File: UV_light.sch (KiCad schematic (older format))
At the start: 89 parts, among them P1 SMD_CONN, P10 SMD_CONN, P2 SMD_CONN, P3 SMD_CONN, P4 SMD_CONN, P5 CONN_01X01, P6 CONN_01X01, P7 SMD_CONN, P8 SMD_CONN, P9 SMD_CONN

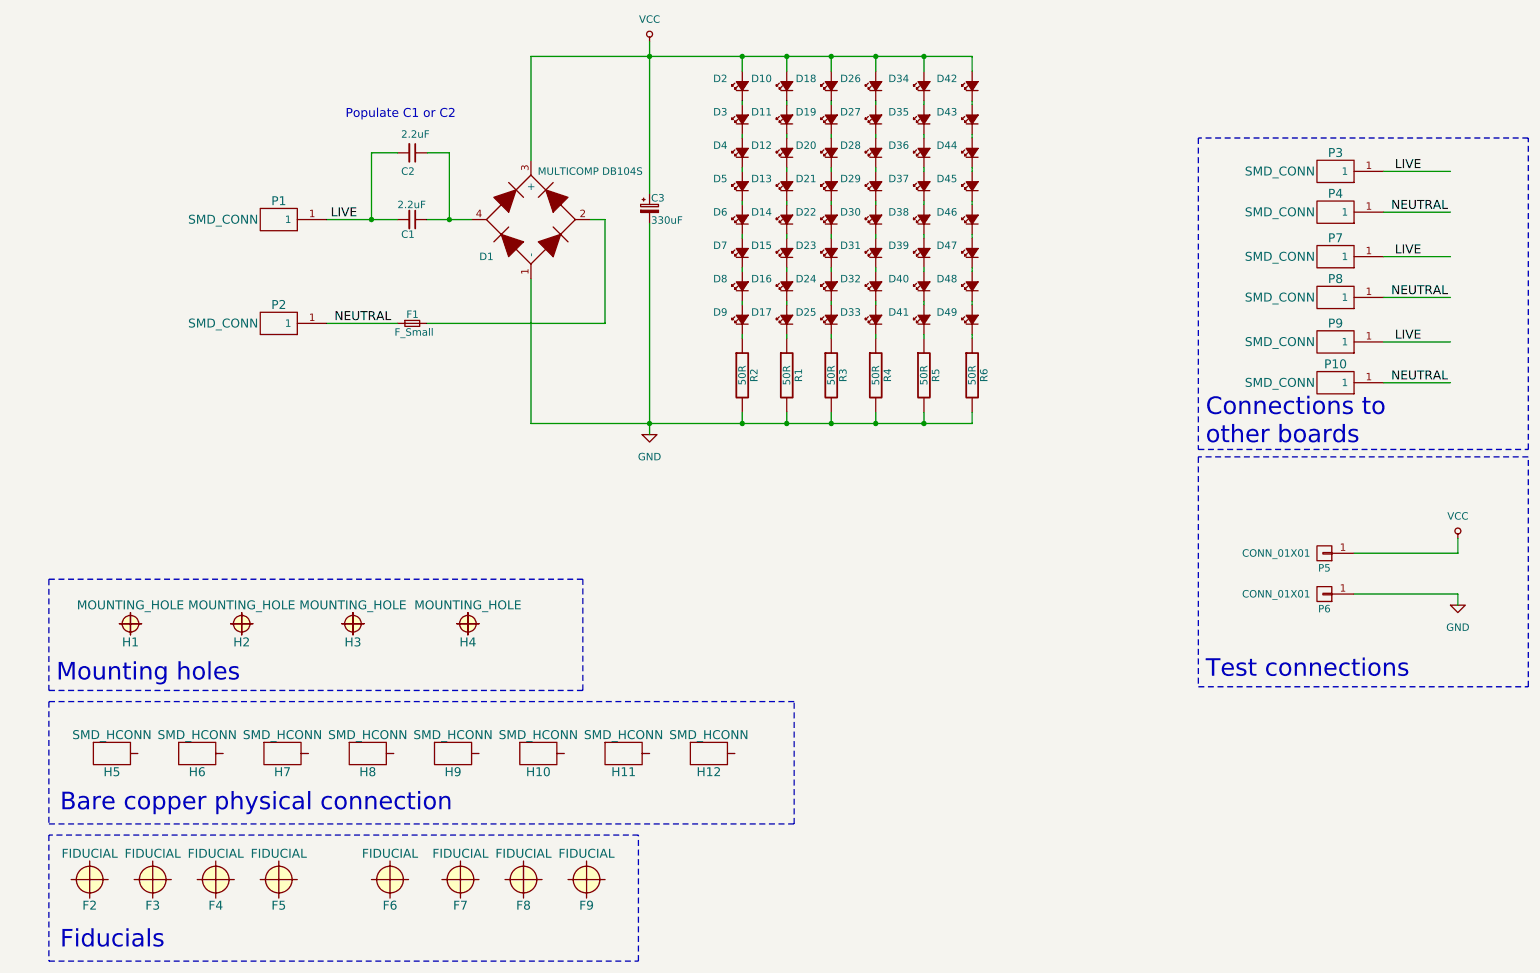
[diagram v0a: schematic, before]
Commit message: Comleting version 2
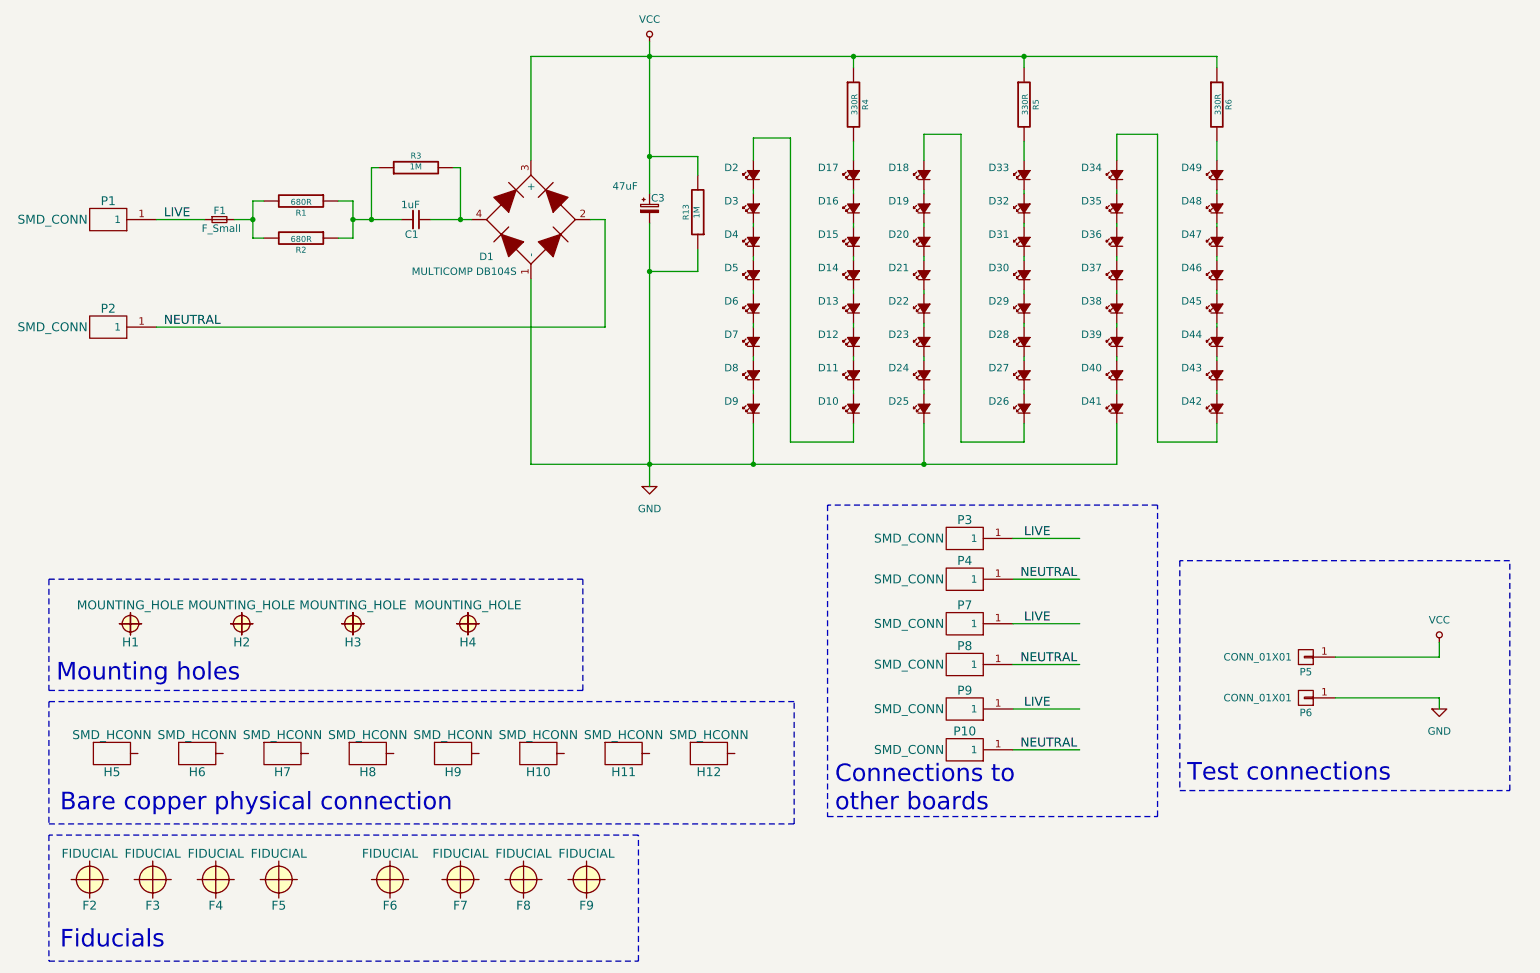
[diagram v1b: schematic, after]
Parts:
- removed C2: 2.2uF, Local:Capacitor_Panasonic_G13, symbol C_Small
- added R13: 1M, Resistors_SMD:R_1206, symbol R
- C1: value 2.2uF -> 1uF; footprint Local:Capacitor_17.5x10x15mm -> Local:Capacitor_film_26.5x10; Farnell code 2581173 -> 2495926; Maker PANASONIC -> KEMET; Maker code ECWFE2W225K -> R71VN41004030K; Type Film Capacitor, ECWFE Series, 2.2 µF, ± 10%, PP (Polypropyl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 -> Film Capacitor, 1 µF, 520 V, R71 Series, ± 10%, Radial Lead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
- C3: value 330uF -> 47uF; footprint Capacitors_SMD:c_elec_8x10 -> Local:Capacitor_Panasonic_G13; Farnell code 2068646 -> 1973389; Maker KEMET -> PANASONIC; Maker code EDK337M010A9MAA -> EEEHA2A470UP; Type SMD Aluminium Electrolytic Capacitor, Radial Can - SMD, 330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 -> SMD Aluminium Electrolytic Capacitor, Radial Can - SMD, 47 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
- P5, P6: footprint Local:TESTPOINT_SMD -> Local:TESTPOINT_SMD_3MM
- R1, R2: value 50R -> 680R; footprint Resistors_SMD:R_0603 -> Resistors_SMD:R_2512; Farnell code (none) -> 2117499; Maker (none) -> TE CONNECTIVITY; Maker code (none) -> 3521680RFT; Type (none) -> SMD Chip Resistor, 680 ohm, 250 V, 2512 [6432 Metric], 2 W,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
- R3: value 50R -> 1M; footprint Resistors_SMD:R_0603 -> Resistors_SMD:R_1206; Farnell code (none) -> 9335781; Maker (none) -> MULTICOMP; Maker code (none) -> MC0125W120611M; Type (none) -> SMD Chip Resistor, Thick Film, 1 Mohm, 200 V, 1206 [3216 Me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
- R4, R5, R6: value 50R -> 330R; footprint Resistors_SMD:R_0603 -> Resistors_SMD:R_1206; Farnell code (none) -> 2332133; Maker (none) -> TE CONNECTIVITY; Maker code (none) -> CRGH1206F330R; Type (none) -> SMD Chip Resistor, Thick Film, 330 ohm, 200 V, 1206 [3216 M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
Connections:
- wire segments 86 -> 103
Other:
- note removed: "Populate C1 or C2"
- moved on the sheet: C1, D10, D11, D12, D13, D14, D15, D16, D17, D2, D3, D4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
